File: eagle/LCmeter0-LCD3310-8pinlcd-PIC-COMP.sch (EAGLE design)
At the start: 36 parts, among them IC1 PIC16F876A, J1 HD44780-4BITLCD44780-8P, J2 PIC-UART, J3 PIC-ICSP, J4 J4, J5 CONN-2P2P/V, J7 CONN-2P2P/V, K2 DS2Y, Q1 20MHz, SW1 PB-1P-1T, T1 BC547

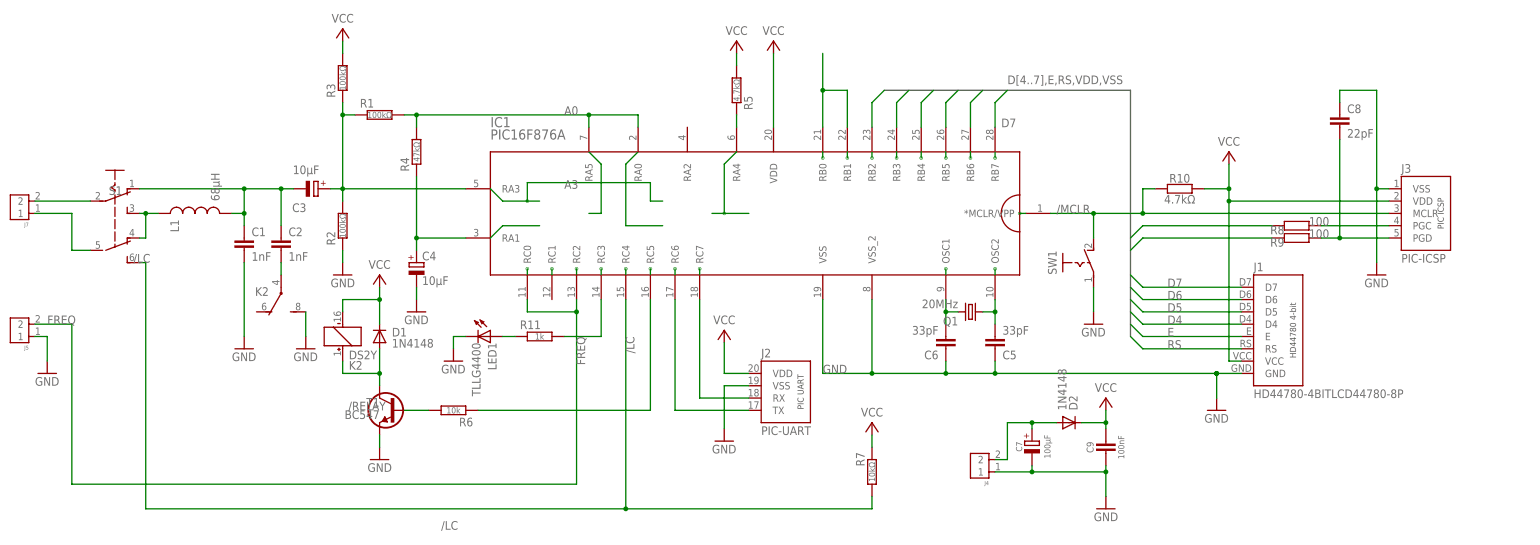
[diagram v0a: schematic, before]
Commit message: ...
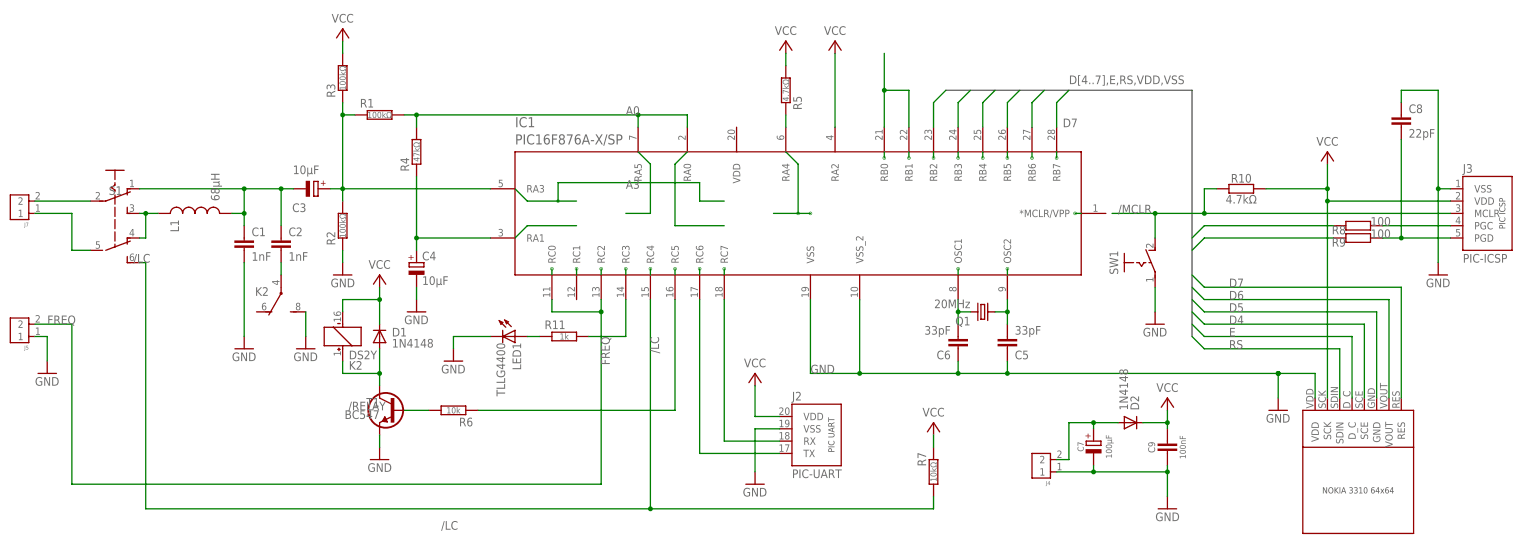
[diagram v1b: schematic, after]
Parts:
- IC1: value PIC16F876A -> PIC16F876A-X/SP; device lc-meter:PIC16F876A-X/SP-COMP-B-A -> mcu:PIC16F876A-X/SP-COMPDIL28-3/V
- J1: value HD44780-4BITLCD44780-8P -> SPI-LCD3310; device pinconn:HD44780-4BITLCD44780-8P -> lcd:NOKIA-3310-64X64SPARKFUN
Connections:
- net /MCLR: no longer IC1.*MCLR/VPP
- net D4: now also J1.SCE; no longer J1.D4
- net D5: now also J1.GND; no longer J1.D5
- net D6: now also J1.VOUT; no longer J1.D6
- net D7: now also J1.RES; no longer J1.D7
- net E: now also J1.D_C; no longer J1.E
- net GND: now also J1.VDD; no longer J1.GND
- net RS: now also J1.SDIN; no longer J1.RS
- net VCC: now also IC1.RA2, J1.SCK; no longer IC1.VDD, J1.VCC
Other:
- moved on the sheet: C5, C6, C7, C8, C9, D2, J2, J3, J4, LED1, Q1, R10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

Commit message: ...
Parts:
- J1: value SPI-LCD3310 -> NOKIA-3310-64X64SPARKFUN
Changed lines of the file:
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@@
 <part name="C8" library="c" deviceset="C" device="050-020X036" value="22pF"/>
 <part name="GND3" library="supply1" deviceset="GND" device=""/>
-<part name="J1" library="lcd" deviceset="NOKIA-3310-64X64" device="SPARKFUN" value="SPI-LCD3310"/>
 <part name="IC1" library="mcu" deviceset="PIC16F876A-X/SP-COMP" device="DIL28-3/V" value="PIC16F876A-X/SP"/>
+<part name="J1" library="lcd" deviceset="NOKIA-3310-64X64" device="SPARKFUN"/>
 </parts>
 <sheets>
@@
 <instance part="C8" gate="G$1" x="261.62" y="45.72"/>
 <instance part="GND3" gate="1" x="269.24" y="12.7"/>
+<instance part="IC1" gate="1" x="137.16" y="25.4"/>
 <instance part="J1" gate="1" x="252.73" y="-31.75" rot="R180"/>
-<instance part="IC1" gate="1" x="137.16" y="25.4"/>
 </instances>
 <busses>
@@
 <junction x="180.34" y="-7.62"/>
 <junction x="236.22" y="-7.62"/>
-<pinref part="J1" gate="1" pin="VDD"/>
 <pinref part="IC1" gate="1" pin="VSS"/>
 <pinref part="IC1" gate="1" pin="VSS_2"/>
-</segment>
-<segment>
+<pinref part="J1" gate="1" pin="VDD"/>
+</segment>
+<segment>
